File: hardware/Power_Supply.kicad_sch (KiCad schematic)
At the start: 74 parts, among them U26 LTC3122HMSE#PBF, U27 LTC3115IDHD-2#WPBF, U28 NCP1117-3.3_SOT223, U29 NCP1117-12_SOT223, U30 LM2990SX-12

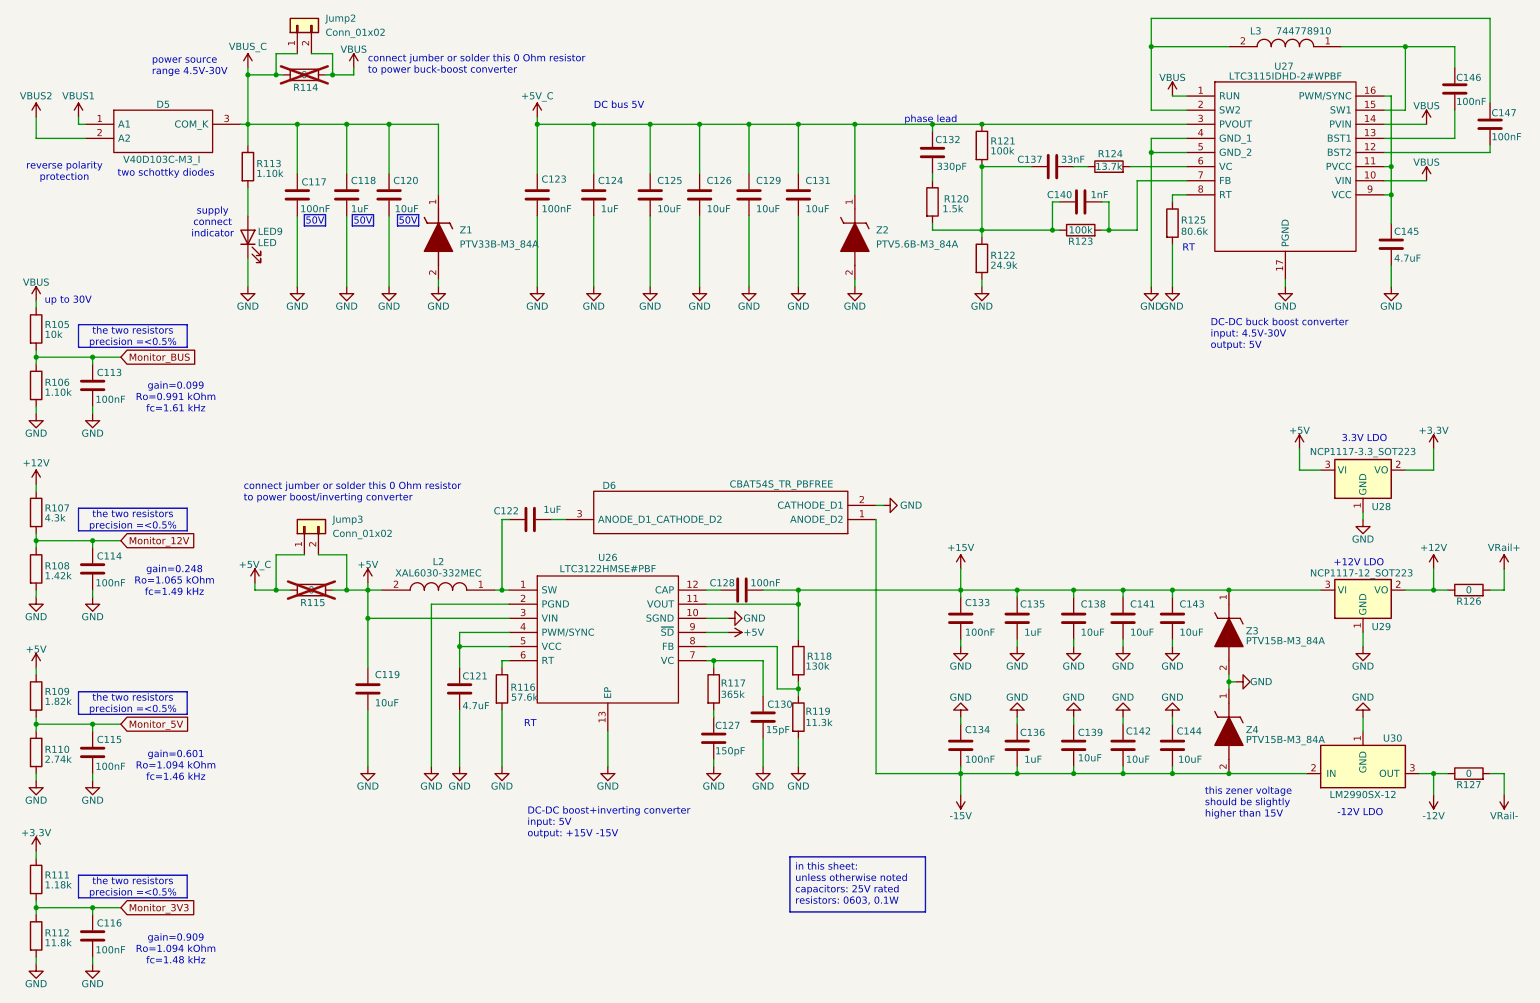
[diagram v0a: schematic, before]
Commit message: Continue BOM + enhance BOM + enhance schematic
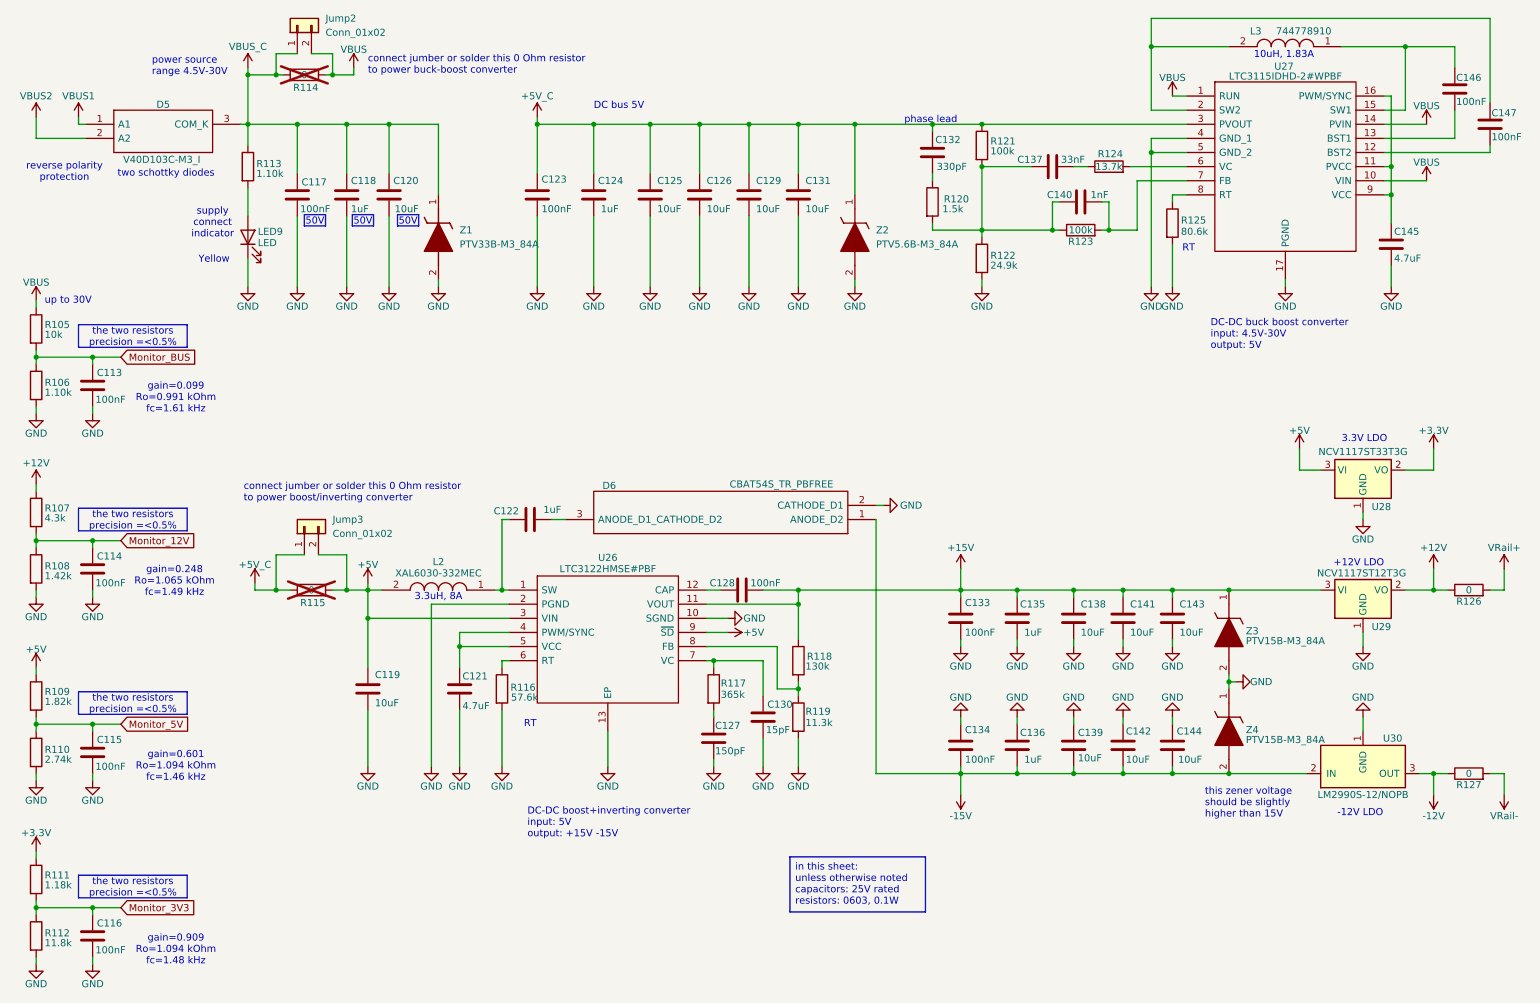
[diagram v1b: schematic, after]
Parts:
- C118, C120, C121, C122, C124, C135, C136, C145: Manufacturer TDK Corporation -> TDK; Manufacturer_Name TDK Corporation -> TDK
- Jump2, Jump3: Manufacturer Harwin Inc. -> Harwin; Manufacturer_Name Harwin Inc. -> Harwin
- L2: Link (none) -> https://www.digikey.com/en/products/detail/coilcraft/XAL603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
- L3: Link (none) -> https://www.digikey.com/en/products/detail/w%C3%BCrth-elekt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
- LED9: Manufacturer_Name (none) -> SunLED
- U26, U27: Link (none) -> https://www.digikey.com/en/products/detail/analog-devices-i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; Manufacturer (none) -> Analog Devices
- U28: value NCP1117-3.3_SOT223 -> NCV1117ST33T3G; Link (none) -> https://www.digikey.com/en/products/detail/onsemi/NCV1117ST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; MPN (none) -> NCV1117ST33T3G; Manufacturer (none) -> Onsemi; Manufacturer_Name (none) -> Onsemi; Manufacturer_Part_Number (none) -> NCV1117ST33T3G
- U29: value NCP1117-12_SOT223 -> NCV1117ST12T3G; Link (none) -> https://www.digikey.com/en/products/detail/onsemi/NCV1117ST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; MPN (none) -> NCV1117ST12T3G; Manufacturer (none) -> Onsemi; Manufacturer_Name (none) -> Onsemi; Manufacturer_Part_Number (none) -> NCV1117ST12T3G
- U30: value LM2990SX-12 -> LM2990S-12/NOPB; Link (none) -> https://www.digikey.com/en/products/detail/texas-instrument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; MPN (none) -> LM2990S-12/NOPB; Manufacturer (none) -> Texas Instruments; Manufacturer_Name (none) -> Texas Instruments; Manufacturer_Part_Number (none) -> LM2990S-12/NOPB
- Z1, Z2, Z3, Z4: Link (none) -> https://www.digikey.com/en/products/detail/vishay-general-s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
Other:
- note added: "10uH, 1.83A"
- note added: "3.3uH, 8A"
- note added: "Yellow"
